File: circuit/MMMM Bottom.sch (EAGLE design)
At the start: 40 parts, among them J4 IN1, J9 POWER_JACKPTH_BREAD

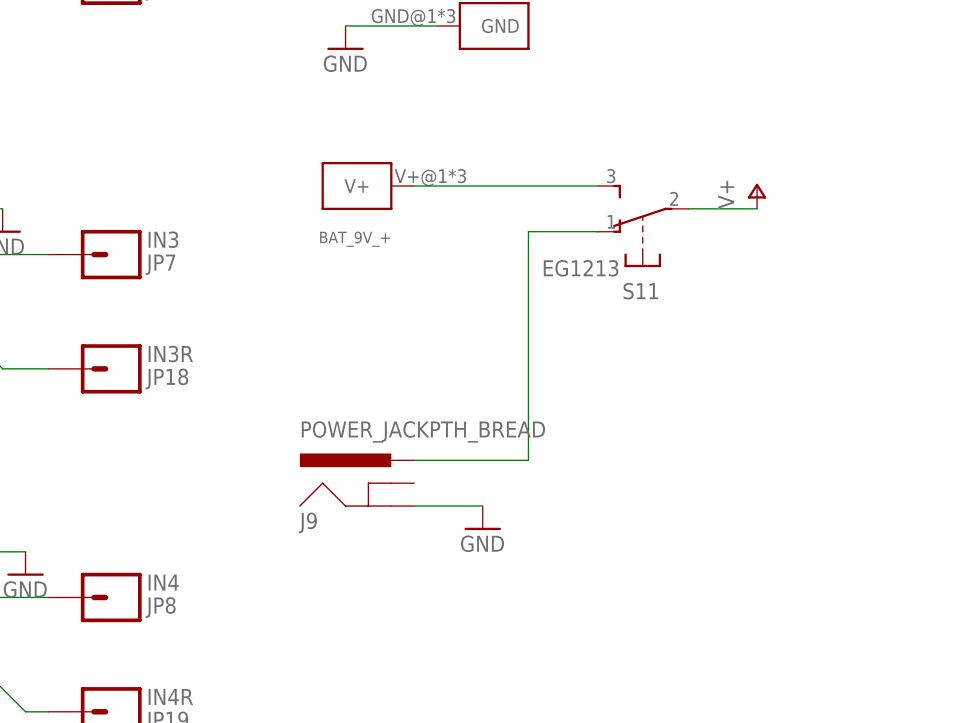
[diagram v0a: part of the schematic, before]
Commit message: Updated
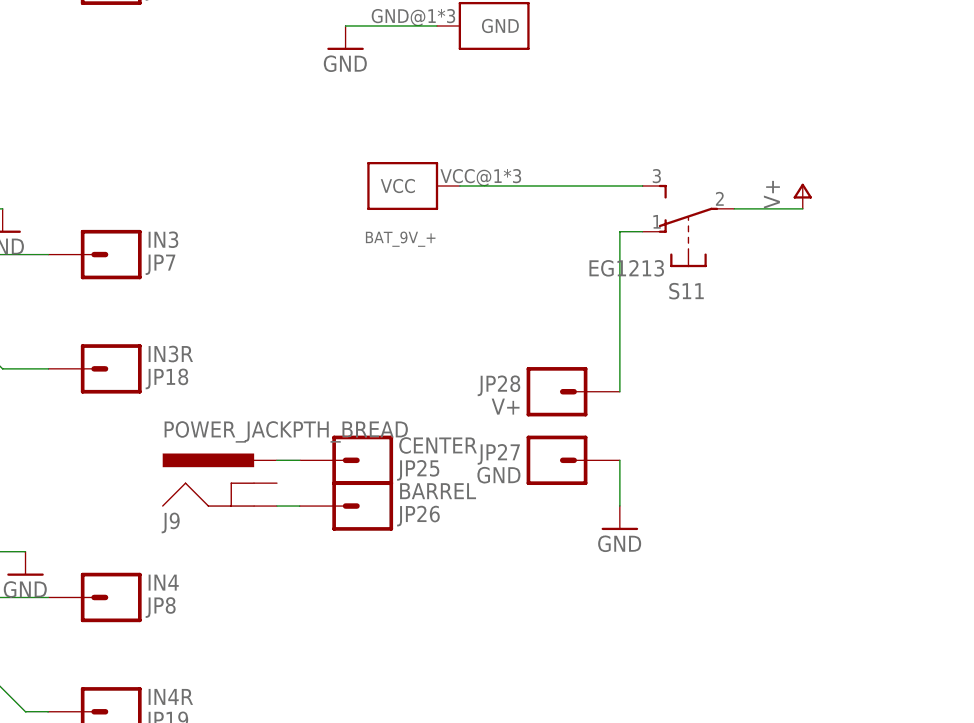
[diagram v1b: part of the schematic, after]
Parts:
- added JP25: CENTER, TOF:HEADER-1X11X01_SIDE_NAME_SML
- added JP26: BARREL, TOF:HEADER-1X11X01_SIDE_NAME_SML
- added JP27: GND, TOF:HEADER-1X11X01_SIDE_NAME_SML
- added JP28: V+, TOF:HEADER-1X11X01_SIDE_NAME_SML
- BAT_9V_+: value KEYSTONE-629+ -> KEYSTONE-637; device kanflo:KEYSTONE-629+ -> kanflo:KEYSTONE-637
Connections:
- new net N$18: J9.PWR, JP25.1
- new net N$19: J9.GND, JP26.1
- net GND: now also JP27.1; no longer J9.GND
- net N$15: now also JP28.1; no longer J9.PWR
- net N$16: now also BAT_9V_+.VCC; no longer BAT_9V_+.V+
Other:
- moved on the sheet: BAT_9V_+, J9, S11
